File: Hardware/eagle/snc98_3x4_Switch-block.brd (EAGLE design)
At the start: 56.4 x 83.2 mm, 67 parts

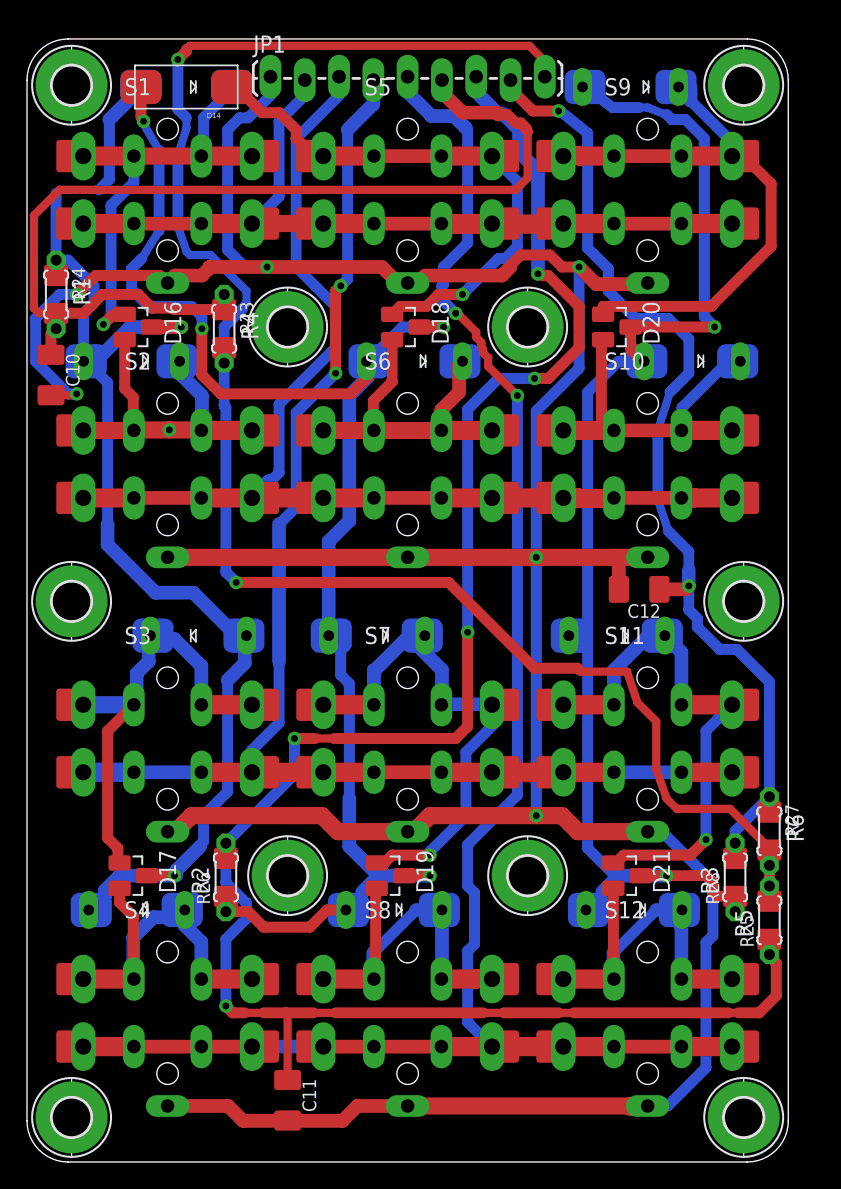
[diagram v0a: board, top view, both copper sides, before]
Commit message: New Hardware Design V0.4
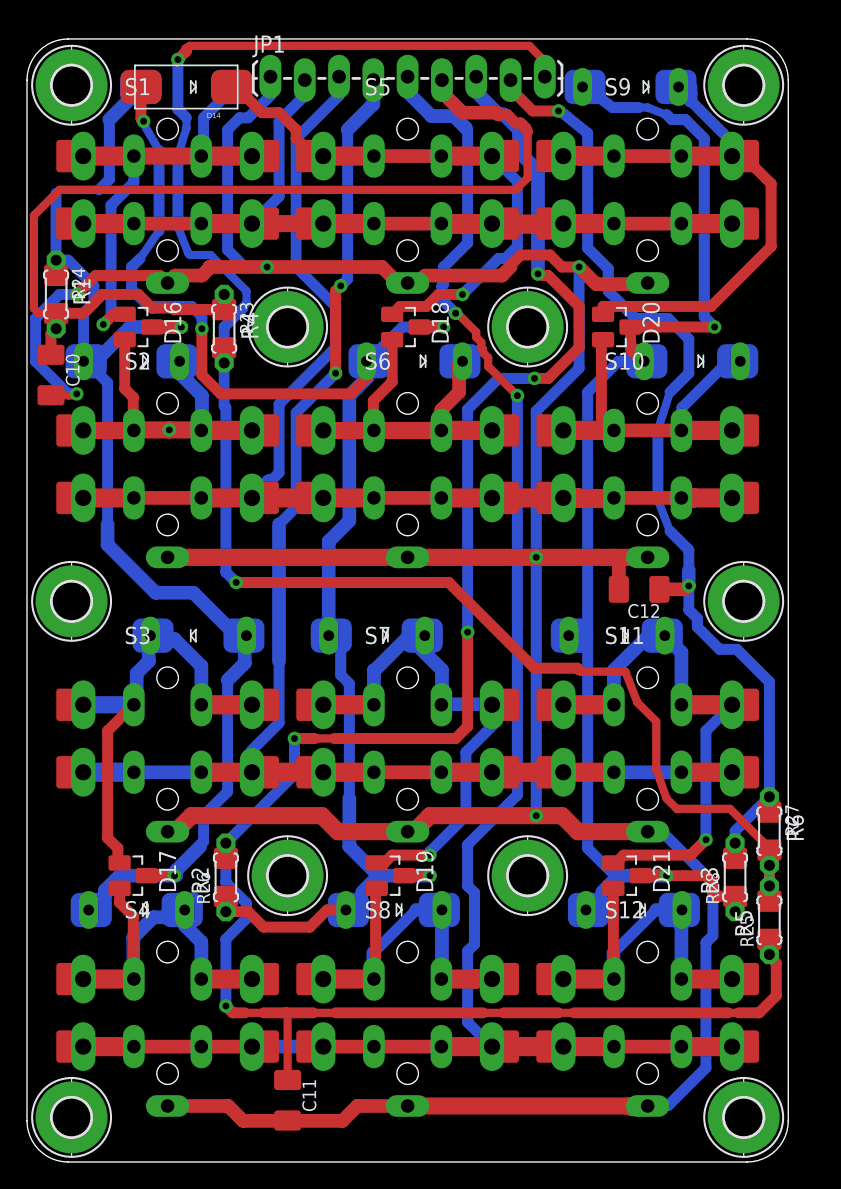
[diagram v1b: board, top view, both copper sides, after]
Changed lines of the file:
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@@
 <setting verticaltext="up"/>
 </settings>
-<grid distance="0.1" unitdist="inch" unit="inch" style="lines" multiple="1" display="yes" altdistance="0.01" altunitdist="inch" altunit="inch"/>
+<grid distance="5" unitdist="mil" unit="mil" style="lines" multiple="1" display="yes" altdistance="0.01" altunitdist="inch" altunit="inch"/>
 <layers>
 <layer number="1" name="Top" color="4" fill="1" visible="yes" active="yes"/>
@@
 <layer number="24" name="bOrigins" color="15" fill="1" visible="yes" active="yes"/>
 <layer number="25" name="tNames" color="7" fill="1" visible="yes" active="yes"/>
-<layer number="26" name="bNames" color="7" fill="1" visible="yes" active="yes"/>
+<layer number="26" name="bNames" color="7" fill="1" visible="no" active="yes"/>
 <layer number="27" name="tValues" color="7" fill="1" visible="no" active="yes"/>
 <layer number="28" name="bValues" color="7" fill="1" visible="no" active="yes"/>
@@
 <wire x1="47.625" y1="57.023" x2="46.736" y2="54.229" width="0.6096" layer="16"/>
 <wire x1="46.736" y1="54.229" x2="46.736" y2="49.022" width="0.8128" layer="16"/>
-<wire x1="46.736" y1="49.022" x2="47.498" y2="46.736" width="0.6096" layer="16"/>
-<wire x1="47.498" y1="46.736" x2="49.022" y2="45.212" width="0.8128" layer="16"/>
-<wire x1="49.022" y1="45.212" x2="49.022" y2="43.815" width="0.8128" layer="16"/>
+<wire x1="46.736" y1="49.022" x2="47.625" y2="46.736" width="0.6096" layer="16"/>
+<wire x1="49.022" y1="45.339" x2="49.022" y2="43.815" width="0.8128" layer="16"/>
 <wire x1="49.022" y1="42.672" x2="49.022" y2="40.894" width="0.8128" layer="16"/>
 <wire x1="49.022" y1="40.894" x2="49.657" y2="40.259" width="0.8128" layer="16"/>
@@
 <wire x1="51.308" y1="37.973" x2="52.578" y2="37.973" width="0.8128" layer="16"/>
 <wire x1="52.578" y1="37.973" x2="54.991" y2="35.56" width="0.8128" layer="16"/>
+<wire x1="47.625" y1="46.736" x2="49.022" y2="45.339" width="0.8128" layer="16"/>
 </signal>
 <signal name="N$21">
@@
 <wire x1="16.256" y1="64.516" x2="13.589" y2="67.183" width="0.6096" layer="16"/>
 <wire x1="13.589" y1="67.183" x2="12.065" y2="67.183" width="0.6096" layer="16"/>
-<wire x1="12.065" y1="67.183" x2="11.811" y2="67.437" width="0.6096" layer="16"/>
+<wire x1="12.065" y1="67.183" x2="11.938" y2="67.31" width="0.6096" layer="16"/>
 <via x="11.176" y="81.661" extent="1-16" drill="0.508"/>
 <wire x1="11.811" y1="82.423" x2="12.065" y2="82.677" width="0.6096" layer="1"/>
@@
 <wire x1="46.609" y1="29.083" x2="46.609" y2="32.639" width="0.6096" layer="1"/>
 <wire x1="46.609" y1="32.639" x2="45.212" y2="34.036" width="0.6096" layer="1"/>
-<wire x1="45.212" y1="34.036" x2="44.45" y2="36.322" width="0.6096" layer="1"/>
-<wire x1="44.45" y1="36.322" x2="41.021" y2="36.322" width="0.6096" layer="1"/>
+<wire x1="45.212" y1="34.036" x2="44.323" y2="36.322" width="0.6096" layer="1"/>
+<wire x1="44.323" y1="36.322" x2="41.021" y2="36.322" width="0.6096" layer="1"/>
 <wire x1="41.021" y1="36.322" x2="40.894" y2="36.449" width="0.6096" layer="1"/>
 <wire x1="40.894" y1="36.449" x2="40.767" y2="36.576" width="0.8128" layer="1"/>
@@
 <via x="15.494" y="42.926" extent="1-16" drill="0.508"/>
 <wire x1="15.494" y1="42.926" x2="31.242" y2="42.926" width="0.8128" layer="1"/>
-<wire x1="11.811" y1="67.437" x2="11.176" y2="69.29820625" width="0.6096" layer="16"/>
+<wire x1="11.938" y1="67.31" x2="11.176" y2="69.29820625" width="0.6096" layer="16"/>
 <wire x1="11.811" y1="82.423" x2="11.811" y2="82.296" width="0.8128" layer="1"/>
 <wire x1="11.811" y1="82.296" x2="11.176" y2="81.661" width="0.8128" layer="1"/>
@@
 <wire x1="8.6995" y1="77.1525" x2="8.636" y2="77.089" width="0.8128" layer="1"/>
 <via x="8.636" y="77.089" extent="1-16" drill="0.508"/>
-<wire x1="7.747" y1="66.167" x2="7.747" y2="64.643" width="0.8128" layer="16"/>
+<wire x1="7.747" y1="66.294" x2="7.747" y2="64.643" width="0.8128" layer="16"/>
 <wire x1="7.747" y1="64.643" x2="9.017" y2="63.373" width="0.8128" layer="16"/>
 <wire x1="9.017" y1="63.373" x2="12.192" y2="63.373" width="0.8128" layer="16"/>
 <wire x1="23.8125" y1="18.669" x2="23.622" y2="18.669" width="0.8128" layer="16"/>
 <wire x1="22.5425" y1="38.989" x2="22.352" y2="38.989" width="0.8128" layer="16"/>
-<wire x1="8.4455" y1="79.629" x2="8.4455" y2="77.4065" width="0.8128" layer="1"/>
+<wire x1="8.4455" y1="79.629" x2="8.4455" y2="77.2795" width="0.8128" layer="1"/>
 <wire x1="8.636" y1="77.089" x2="8.636" y2="76.8985" width="0.6096" layer="16"/>
 <wire x1="8.636" y1="76.8985" x2="9.779" y2="74.93" width="0.6096" layer="16"/>
 <wire x1="9.779" y1="74.93" x2="9.779" y2="68.961" width="0.8128" layer="16"/>
-<wire x1="8.509" y1="66.929" x2="7.747" y2="66.167" width="0.8128" layer="16"/>
-<wire x1="8.509" y1="66.929" x2="9.779" y2="68.961" width="0.6096" layer="16"/>
-<wire x1="8.4455" y1="77.4065" x2="8.636" y2="77.089" width="0.8128" layer="1"/>
+<wire x1="8.382" y1="66.929" x2="9.779" y2="68.961" width="0.6096" layer="16"/>
 <wire x1="24.8285" y1="20.0025" x2="24.8285" y2="19.685" width="0.8128" layer="16"/>
 <wire x1="24.8285" y1="19.685" x2="23.8125" y2="18.669" width="0.8128" layer="16"/>
@@
 <wire x1="23.876" y1="26.924" x2="23.876" y2="23.368" width="1.016" layer="16"/>
 <wire x1="23.876" y1="23.368" x2="26.035" y2="21.209" width="1.016" layer="16"/>
+<wire x1="8.636" y1="77.089" x2="8.4455" y2="77.2795" width="0.8128" layer="1"/>
+<wire x1="8.382" y1="66.929" x2="7.747" y2="66.294" width="0.8128" layer="16"/>
 </signal>
 <signal name="A_3">

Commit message: snc98_main_cpu V1.0
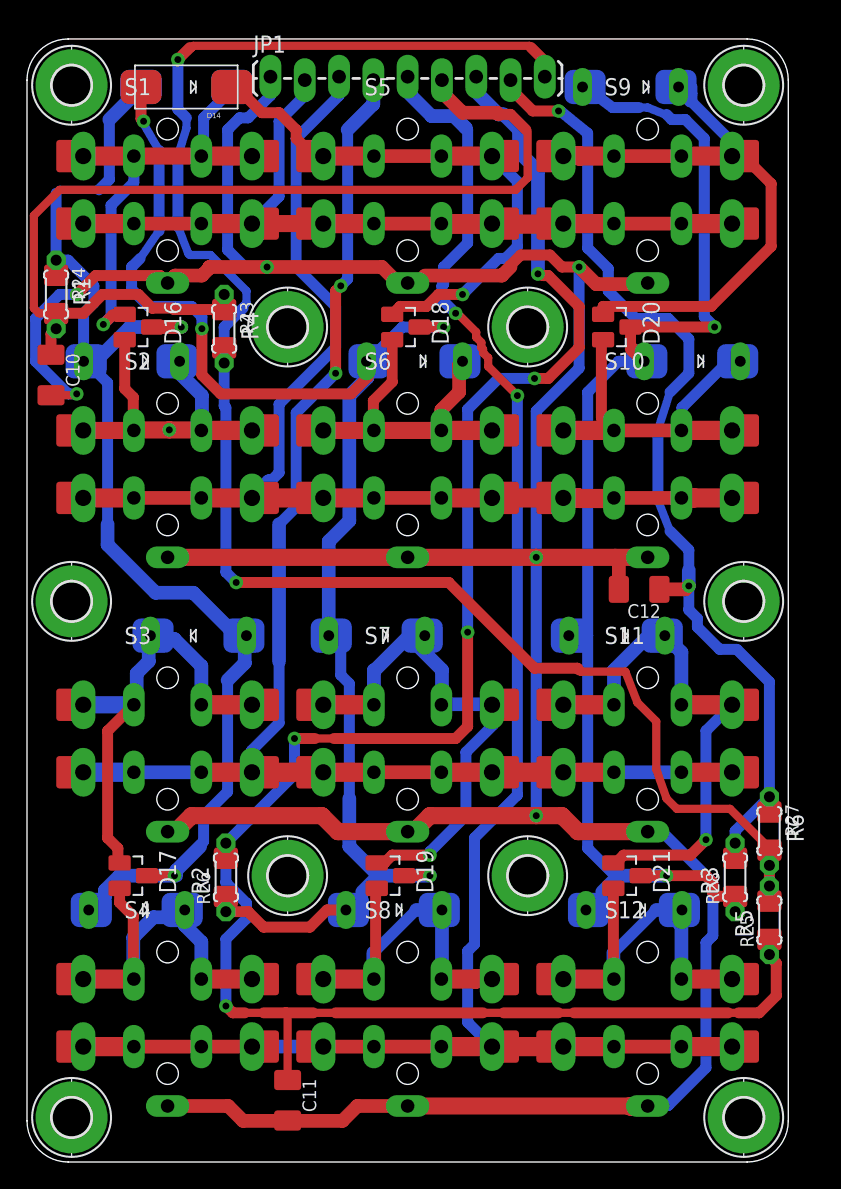
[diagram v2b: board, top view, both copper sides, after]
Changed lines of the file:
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@@
 <dimension x1="10.414" y1="11.049" x2="10.414" y2="72.009" x3="-9.398" y3="41.529" textsize="1.778" textratio="15" layer="47" visible="yes"/>
 <dimension x1="10.414" y1="11.049" x2="45.974" y2="11.049" x3="28.194" y3="-9.652" textsize="1.778" textratio="15" layer="47" visible="yes"/>
-<dimension x1="0" y1="0" x2="56.388" y2="0" x3="28.194" y3="-18.923" textsize="1.778" textratio="15" layer="47"/>
-<dimension x1="3.302" y1="3.302" x2="53.086" y2="3.302" x3="28.194" y3="-13.97" textsize="1.778" textratio="15" layer="47"/>
-<dimension x1="53.086" y1="3.302" x2="53.086" y2="41.529" x3="60.96" y3="22.4155" textsize="1.778" textratio="15" layer="47"/>
-<dimension x1="53.086" y1="3.302" x2="53.086" y2="79.756" x3="66.294" y3="41.529" textsize="1.778" textratio="15" layer="47"/>
+<dimension x1="0" y1="0" x2="56.388" y2="0" x3="28.194" y3="-18.923" textsize="1.778" textratio="15" layer="47" visible="yes"/>
+<dimension x1="3.302" y1="3.302" x2="53.086" y2="3.302" x3="28.194" y3="-13.97" textsize="1.778" textratio="15" layer="47" visible="yes"/>
+<dimension x1="53.086" y1="3.302" x2="53.086" y2="41.529" x3="60.96" y3="22.4155" textsize="1.778" textratio="15" layer="47" visible="yes"/>
+<dimension x1="53.086" y1="3.302" x2="53.086" y2="79.756" x3="66.294" y3="41.529" textsize="1.778" textratio="15" layer="47" visible="yes"/>
 <wire x1="3.048" y1="83.185" x2="0" y2="80.137" width="0" layer="20" curve="90"/>
 <wire x1="56.388" y1="80.137" x2="53.34" y2="83.185" width="0" layer="20" curve="90"/>
 <wire x1="0" y1="3.048" x2="3.048" y2="0" width="0" layer="20" curve="90"/>
 <wire x1="53.34" y1="0" x2="56.388" y2="3.048" width="0" layer="20" curve="90"/>
+<dimension x1="10.414" y1="72.009" x2="10.414" y2="80.264" x3="-9.398" y3="76.1365" textsize="1.778" textratio="15" layer="47" visible="yes"/>
 </plain>
 <attributes>
@@
 <wire x1="31.877" y1="62.865" x2="33.274" y2="61.468" width="0.6096" layer="1"/>
 <wire x1="30.734" y1="63.881" x2="31.75" y2="62.865" width="0.8128" layer="16"/>
-<wire x1="32.639" y1="20.447" x2="32.639" y2="23.495" width="0.8128" layer="16"/>
-<wire x1="36.322" y1="27.178" x2="32.639" y2="23.495" width="0.8128" layer="16"/>
-<wire x1="32.639" y1="20.447" x2="33.147" y2="19.939" width="0.8128" layer="16"/>
-<wire x1="33.147" y1="19.939" x2="33.147" y2="16.129" width="0.8128" layer="16"/>
+<wire x1="33.147" y1="24.003" x2="33.147" y2="16.129" width="0.8128" layer="16"/>
 <wire x1="33.147" y1="16.129" x2="32.639" y2="15.621" width="0.8128" layer="16"/>
 <wire x1="32.639" y1="15.621" x2="32.639" y2="10.354" width="0.8128" layer="16"/>
@@
 <wire x1="12.914" y1="8.549" x2="16.664" y2="8.549" width="1.016" layer="1"/>
 <wire x1="21.944" y1="8.549" x2="25.694" y2="8.549" width="1.016" layer="1"/>
+<wire x1="36.322" y1="27.178" x2="33.147" y2="24.003" width="0.8128" layer="16"/>
 </signal>
 <signal name="C3">
@@
 <wire x1="32.258" y1="77.724" x2="34.798" y2="77.724" width="1.016" layer="1"/>
 <wire x1="34.798" y1="77.724" x2="34.925" y2="77.597" width="1.016" layer="1"/>
-<wire x1="34.925" y1="77.597" x2="35.56" y2="77.597" width="0.8128" layer="1"/>
-<wire x1="35.56" y1="77.597" x2="36.195" y2="76.962" width="0.8128" layer="1"/>
-<wire x1="36.195" y1="76.962" x2="36.576" y2="76.962" width="0.8128" layer="1"/>
-<wire x1="36.576" y1="76.962" x2="36.957" y2="76.581" width="0.8128" layer="1"/>
-<wire x1="36.957" y1="76.581" x2="36.957" y2="76.454" width="0.8128" layer="1"/>
-<wire x1="36.957" y1="76.454" x2="37.084" y2="76.327" width="0.8128" layer="1"/>
+<wire x1="34.925" y1="77.597" x2="35.814" y2="77.597" width="0.8128" layer="1"/>
+<wire x1="35.814" y1="77.597" x2="36.957" y2="76.454" width="0.8128" layer="1"/>
 <wire x1="37.084" y1="76.327" x2="37.084" y2="72.898" width="0.6096" layer="1"/>
 <wire x1="37.084" y1="72.898" x2="36.195" y2="72.009" width="0.6096" layer="1"/>
@@
 <wire x1="5.588" y1="64.262" x2="4.191" y2="62.865" width="0.8128" layer="1"/>
 <wire x1="4.191" y1="62.865" x2="1.651" y2="62.865" width="0.8128" layer="1"/>
+<wire x1="36.957" y1="76.454" x2="37.084" y2="76.454" width="0.254" layer="1"/>
+<wire x1="37.084" y1="76.454" x2="37.084" y2="76.327" width="0.254" layer="1"/>
 </signal>
 <signal name="GND">
@@
 <wire x1="12.065" y1="67.183" x2="11.938" y2="67.31" width="0.6096" layer="16"/>
 <via x="11.176" y="81.661" extent="1-16" drill="0.508"/>
-<wire x1="11.811" y1="82.423" x2="12.065" y2="82.677" width="0.6096" layer="1"/>
 <wire x1="38.481" y1="81.407" x2="38.481" y2="80.518" width="0.8128" layer="1"/>
 <wire x1="38.481" y1="80.518" x2="38.354" y2="80.391" width="0.8128" layer="1"/>
 <wire x1="11.176" y1="69.342" x2="11.176" y2="69.29820625" width="0.6096" layer="16"/>
-<wire x1="37.211" y1="82.677" x2="38.481" y2="81.407" width="0.6096" layer="1"/>
-<wire x1="37.211" y1="82.677" x2="12.065" y2="82.677" width="0.6096" layer="1"/>
+<wire x1="37.211" y1="82.677" x2="12.319" y2="82.677" width="0.6096" layer="1"/>
 <wire x1="11.176" y1="81.661" x2="11.176" y2="77.978" width="0.8128" layer="16"/>
 <wire x1="11.176" y1="77.978" x2="11.811" y2="77.343" width="0.8128" layer="16"/>
@@
 <wire x1="15.494" y1="42.926" x2="31.242" y2="42.926" width="0.8128" layer="1"/>
 <wire x1="11.938" y1="67.31" x2="11.176" y2="69.29820625" width="0.6096" layer="16"/>
-<wire x1="11.811" y1="82.423" x2="11.811" y2="82.296" width="0.8128" layer="1"/>
-<wire x1="11.811" y1="82.296" x2="11.176" y2="81.661" width="0.8128" layer="1"/>
+<wire x1="12.065" y1="82.55" x2="11.176" y2="81.661" width="0.8128" layer="1"/>
+<wire x1="12.192" y1="82.55" x2="11.938" y2="82.296" width="0.6096" layer="1"/>
+<wire x1="38.481" y1="81.407" x2="37.338" y2="82.55" width="0.8128" layer="1"/>
+<wire x1="37.338" y1="82.55" x2="37.211" y2="82.677" width="0.6096" layer="1"/>
+<wire x1="12.319" y1="82.677" x2="12.192" y2="82.55" width="0.6096" layer="1"/>
+<wire x1="12.192" y1="82.55" x2="12.065" y2="82.55" width="0.6096" layer="1"/>
 </signal>
 <signal name="A_1">
